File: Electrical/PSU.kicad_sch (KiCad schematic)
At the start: 104 parts, among them IC2 SiC437AED-T1-GE3, J15 Conn_01x03_Pin, J16 USB_C_Receptacle_USB2.0, Q10 2N7002, Q8 2N7002, Q9 2N7002, SW1 SW_Push, U12 ADP1715ARMZ-R7, U13 HT7533, U14 CH224Q_C46061833, U15 SY8253ADC, U16 SY8253ADC, U17 ADP1715ARMZ-R7, U6 SY8253ADC

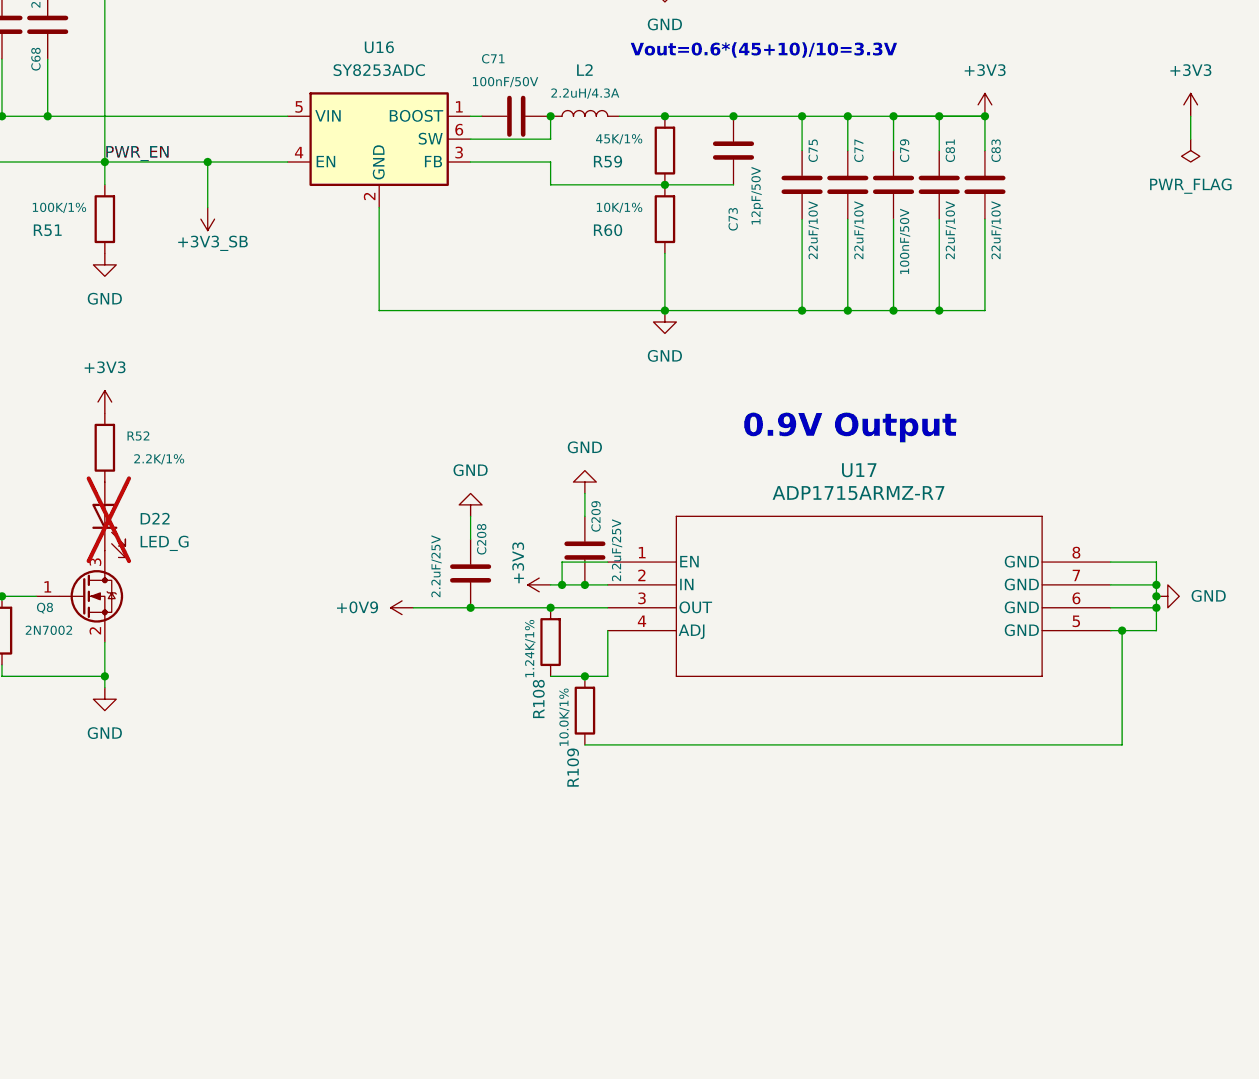
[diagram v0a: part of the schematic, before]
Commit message: Revert "update 0.9v regulator"
This reverts commit 20026994f1eba6e61bd33e858c390714c2ea728b.
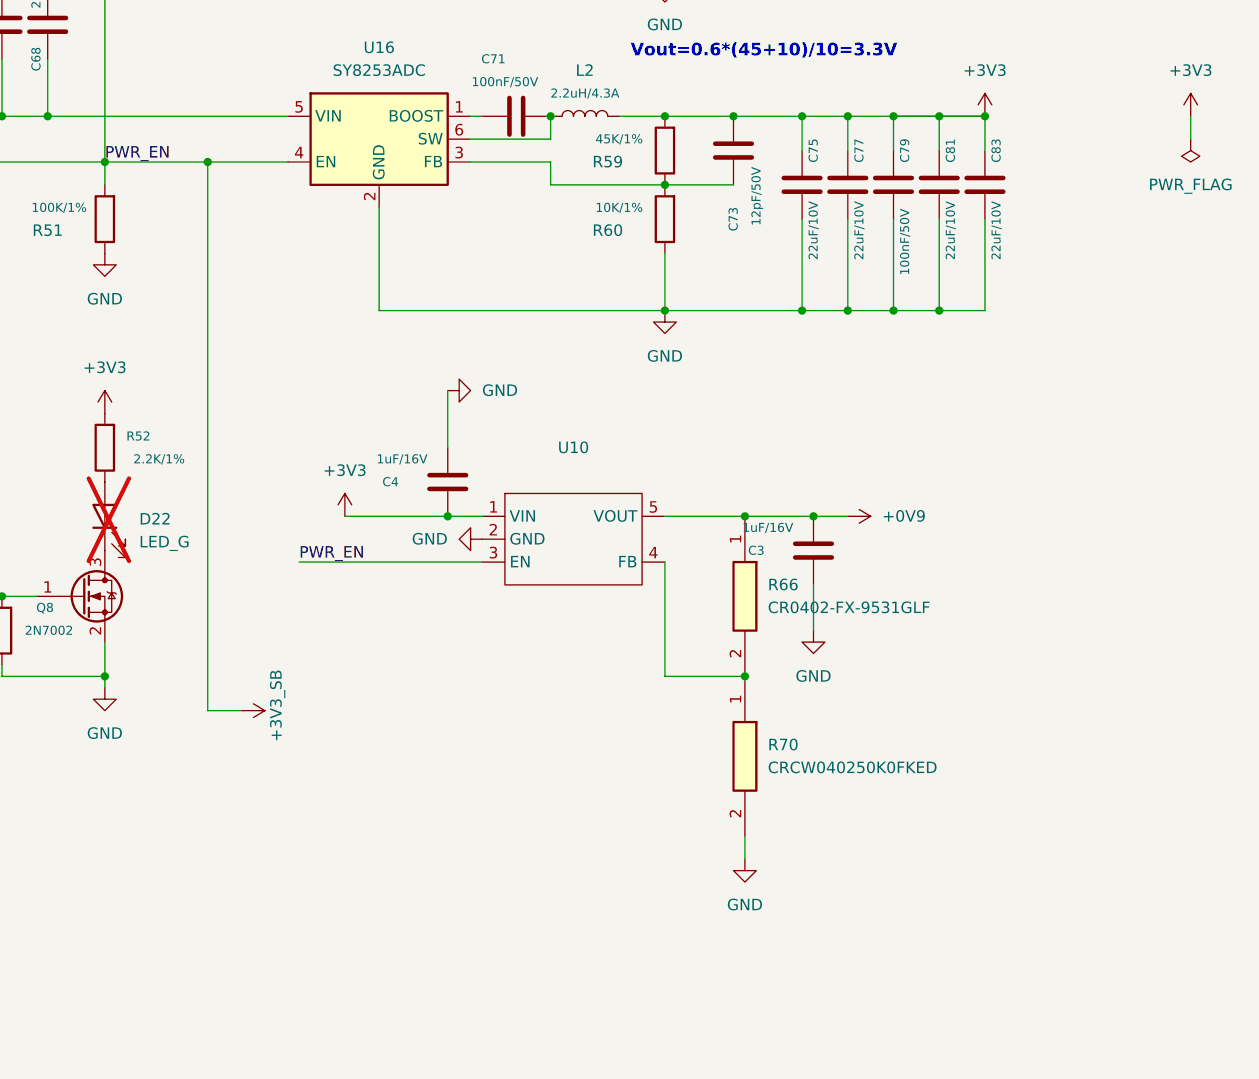
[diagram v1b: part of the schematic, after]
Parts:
- removed C208, C209: 2.2uF/25V, Capacitor_SMD:C_0603_1608Metric_Pad1.08x0.95mm_HandSolder, symbol Device:C
- removed R108: 1.24K/1%, Resistor_SMD:R_0201_0603Metric_Pad0.64x0.40mm_HandSolder, symbol Device:R
- removed R109: 10.0K/1%, Resistor_SMD:R_0201_0603Metric_Pad0.64x0.40mm_HandSolder, symbol Device:R
- removed U17: ADP1715ARMZ-R7, 1v ldo:RM_8_ADI, symbol 1v ldo:ADP1715ARMZ-R7
- added C3, C4: 1uF/16V, A_HDJ_Library:C_0402_1005Metric, symbol Device:C
- added R66: CR0402-FX-9531GLF, RESC1005X40N, symbol 9.53k resis:CR0402-FX-9531GLF
- added R70: CRCW040250K0FKED, RESC1005X40N, symbol 50k resis:CRCW040250K0FKED
- added U10: (no value), Package_TO_SOT_SMD:SOT-23-5, symbol ldo:BL8079AGCB5TR
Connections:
- net +0V9: now also C3.1, R66.1, U10.5 (VOUT)
- net +3V3: now also C4.2, U10.1 (VIN)
- net +3V3_SB: now also U10.3 (EN)
- net GND: now also C3.2, C4.1, R70.2, U10.2 (GND)
- new net: R66.2, R70.1, U10.4 (FB)
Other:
- note removed: "0.9V Output"
